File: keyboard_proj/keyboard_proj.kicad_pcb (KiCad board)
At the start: 2 copper layers, 72.7 x 56.6 mm, 74 parts, among them IC1 DW01A-G, IC2 TP4056-42-ESOP8, IC3 LD1117DT12CTR, IC4 USBLC6-4SC6, J1 Conn_02x04_Odd_Even, J2 Conn_01x32, Q1 FS8205A, Q2 2N7002, SW1 SW_Push, U1 STM32WB55CGU6, U2 DLF162500LT-5028A1, U3 DP2032K76812001, U4 SX3B32.000F1210F30, U5 918-418K2023S40026, U6 XL9555QF24, U7 SK12D07VG5, U9 1.0K-ES-4PWB

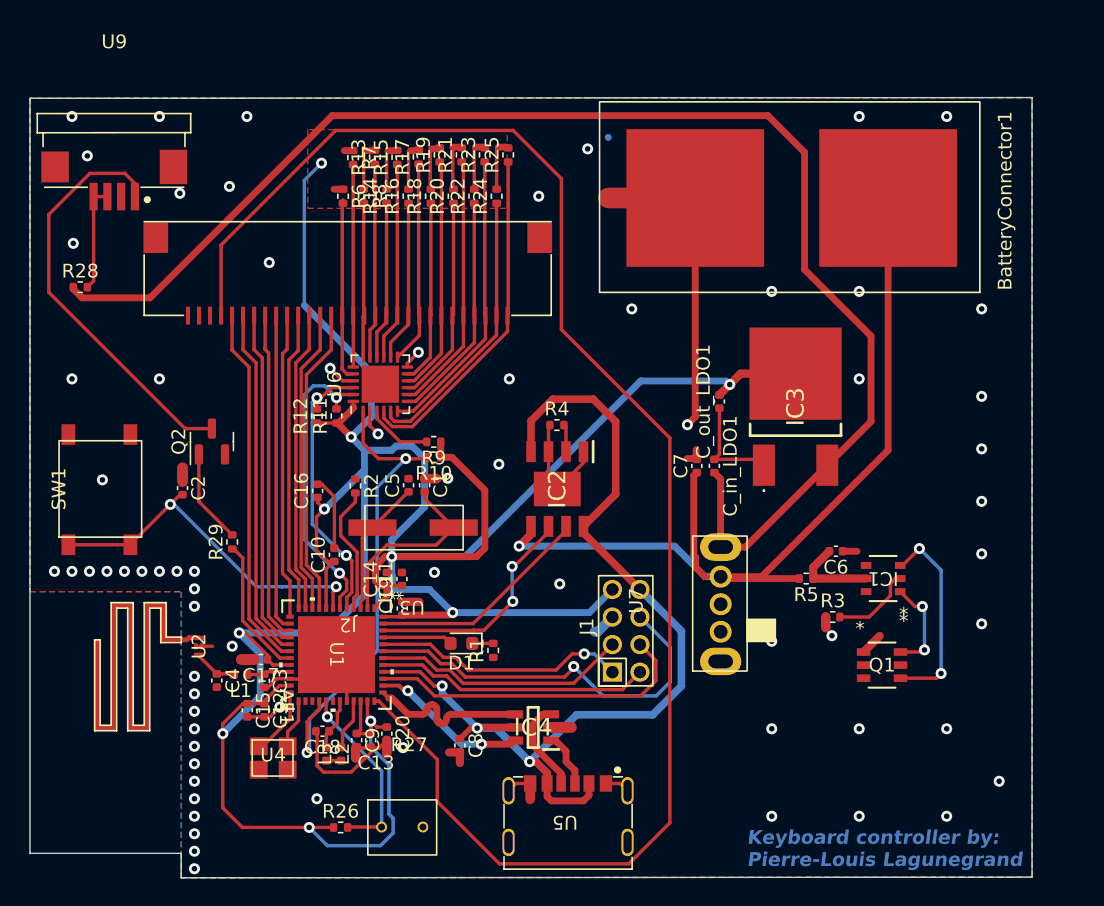
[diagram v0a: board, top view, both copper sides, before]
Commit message: PCB bien avancé, presque fini mais je dois selectionner des pieces de jlcpcb pour baisser les couts
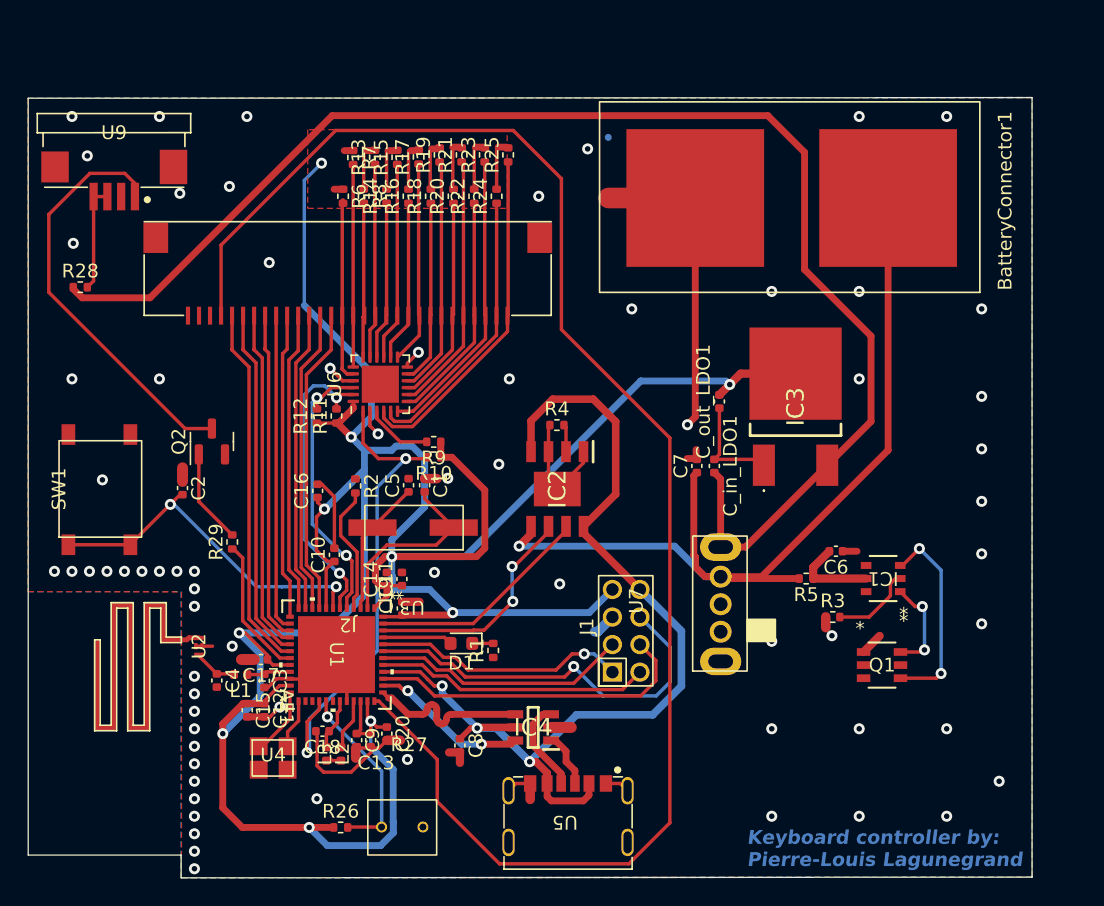
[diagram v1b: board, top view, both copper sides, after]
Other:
- board size 72.7 x 56.6 mm -> 72.9 x 56.6 mm
